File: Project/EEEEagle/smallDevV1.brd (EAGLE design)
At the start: 25.4 x 54 mm, 25 parts, among them IC1 TLC272D

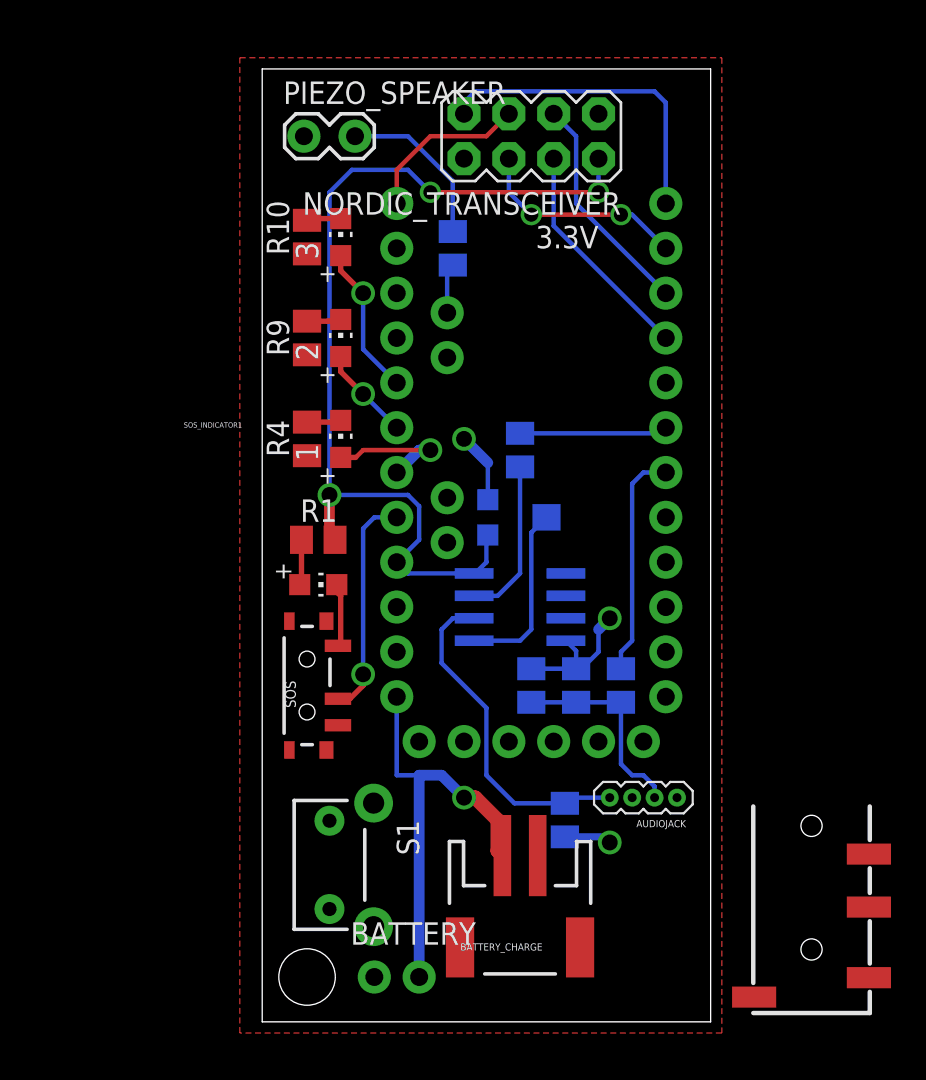
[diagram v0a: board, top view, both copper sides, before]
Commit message: commit yo
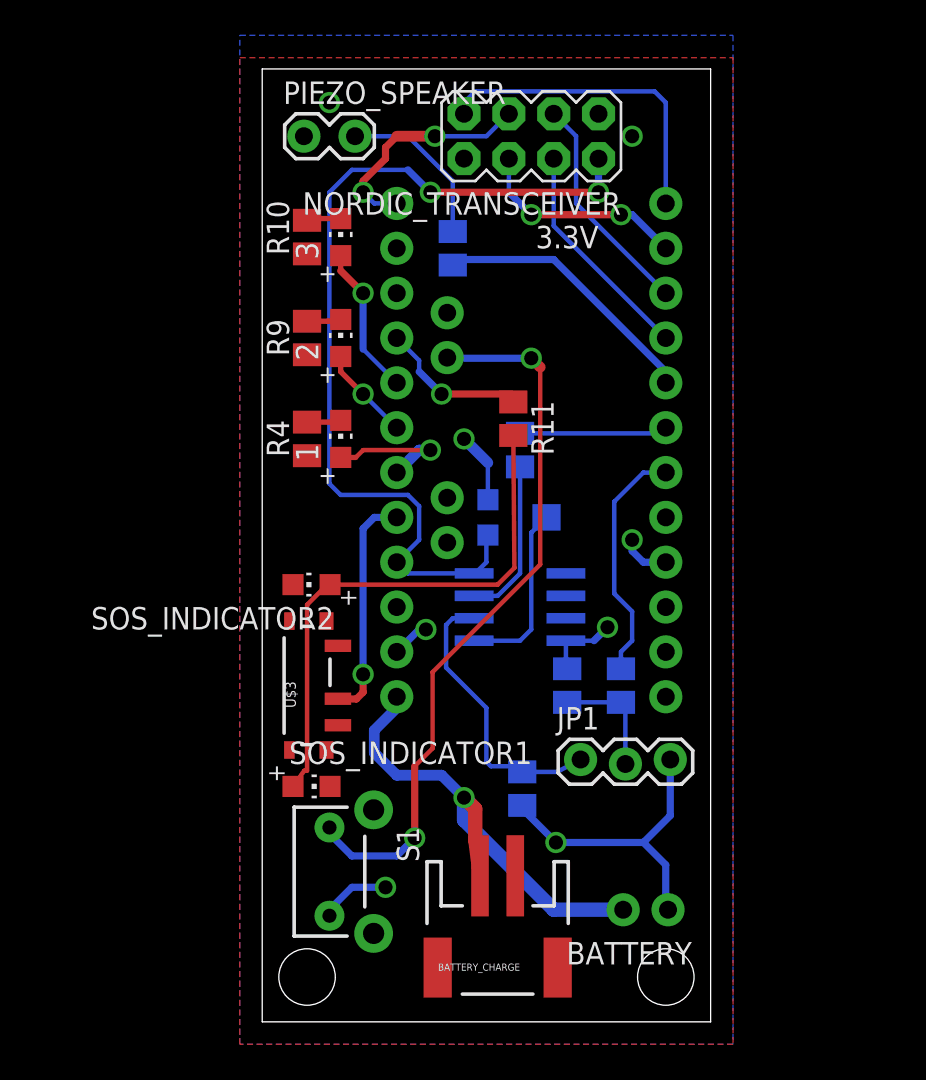
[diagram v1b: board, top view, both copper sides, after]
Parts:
- removed AUDIOJACK: (no value), myLibrary:1X04-1.27MM
- removed R1: 1K, adafruit:M0805
- removed R7: 20K, adafruit:M0805
- removed SOS: (no value), SparkFun-Electromechanical:SWITCH-SPST-SMD-A
- removed U$2: AUDIO-JACK3, SparkFun-Connectors:AUDIO-JACK-TRRS-SMD
- added JP1: Microphone, SparkFun-Connectors:1X03_LOCK
- added R11: 1K, adafruit:M0805
- added SOS_INDICATOR2: (no value), adafruit:CHIP-LED0805
- added U$3: SWITCH_SPDT, myLibrary:SWITCH-SPST-SMD-A-NOTHRUHOLE
- 3.3V: device SparkFun-Boards:ARDUINO_PRO_MINI -> myLibrary:ARDUINO_PRO_MINI_NO_PROGRAMMING_HEADER
- U$1: value (none) -> 10K
- moved BATTERY 17.1 mm to (23.0, 6.35), turned to 180 degrees
- moved SOS_INDICATOR1 11.4 mm to (2.79, 13.3)
- moved R2 3.00 mm to (14.7, 13.2)
- moved R5 2.03 mm to (17.3, 19.1)
- moved BATTERY_CHARGE 1.71 mm to (13.3, 4.57)
- moved S1 0.38 mm to (3.81, 8.51)
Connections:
- removed net BLEH: 3.3V.5
- removed net N$10: R1.1, SOS_INDICATOR1.A
- removed net N$11: 3.3V.16
- removed net N$12: 3.3V.15
- removed net N$2: AUDIOJACK.4, IC1.6, R2.1
- removed net N$5: 3.3V.2
- removed net N$7: AUDIOJACK.2, R5.1, R6.2, R7.2
- removed net N$9: SOS.3, SOS_INDICATOR1.C
- new net LED: 3.3V.16, R11.1
- new net MICROPHONE: JP1.2, R5.1, R6.2
- new net N$1: R11.2, SOS_INDICATOR1.A, SOS_INDICATOR2.A
- new net SPEAKER_R: IC1.6, JP1.1, R2.1
- net BUTTON: now also 3.3V.A7
- net GND: now also JP1.3, SOS_INDICATOR1.C, SOS_INDICATOR2.C, U$3.1; no longer AUDIOJACK.1, R7.1, SOS.1
- net SPEAKER: now also 3.3V.8; no longer 3.3V.A6
- net SWITCH: now also U$3.2; no longer SOS.2
- net VCC: no longer R1.2
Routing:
- net BUTTON: track 0.00 -> 41.2 mm, vias 0 -> 2
- net N$1: track 0.00 -> 30.7 mm
- net GND: track 14.9 -> 34.9 mm, vias 3 -> 8
- net N$2: track 19.2 -> 0.00 mm
- net SPEAKER_R: track 0.00 -> 16.2 mm
- net SPEAKER: track 2.83 -> 15.9 mm
- net N$7: track 11.6 -> 0.00 mm
- net LED: track 0.00 -> 8.68 mm, vias 0 -> 1
- net MICROPHONE: track 0.00 -> 6.65 mm
- net N$9: track 4.21 -> 0.00 mm
- net SCK: track 9.57 -> 13.0 mm, vias 0 -> 2
- net VCC: track 54.2 -> 51.2 mm, vias 3 -> 2
- net N$10: track 2.58 -> 0.00 mm
- net BATT_VCC: track 24.8 -> 26.9 mm
- net TX: track 12.9 -> 13.8 mm
- added copper zone on layer 16, net GND
